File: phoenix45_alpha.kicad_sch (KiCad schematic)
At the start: 115 parts, among them J1 AVR-ISP-6, SW1 SW_PUSH, SW2 SW_PUSH, U1 SRV05-4, U3 ATmega32U4-M, X1 Crystal_GND24_Small

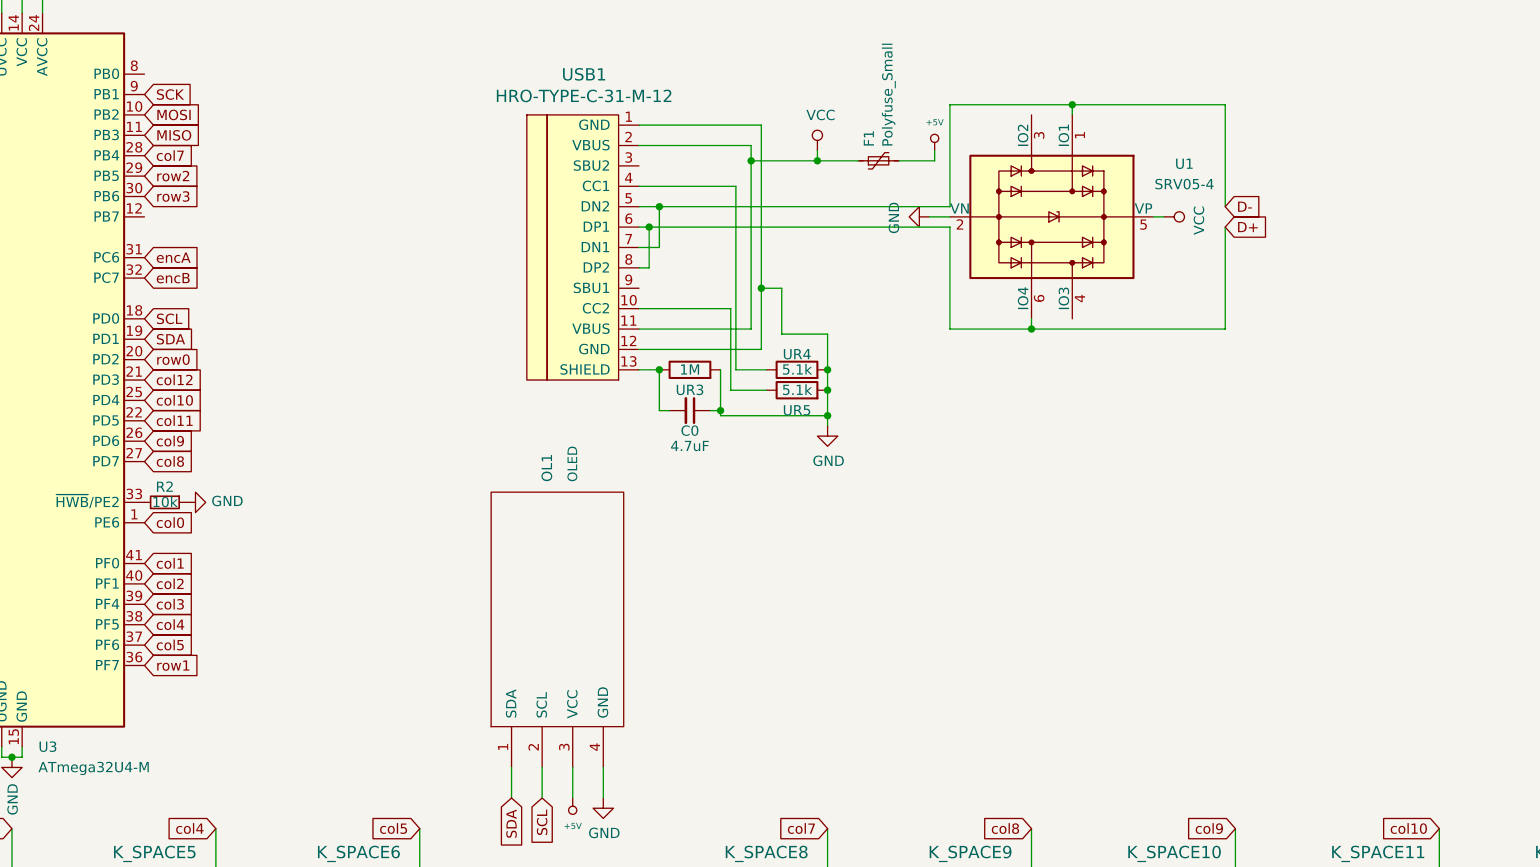
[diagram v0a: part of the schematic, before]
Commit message: trackpoint
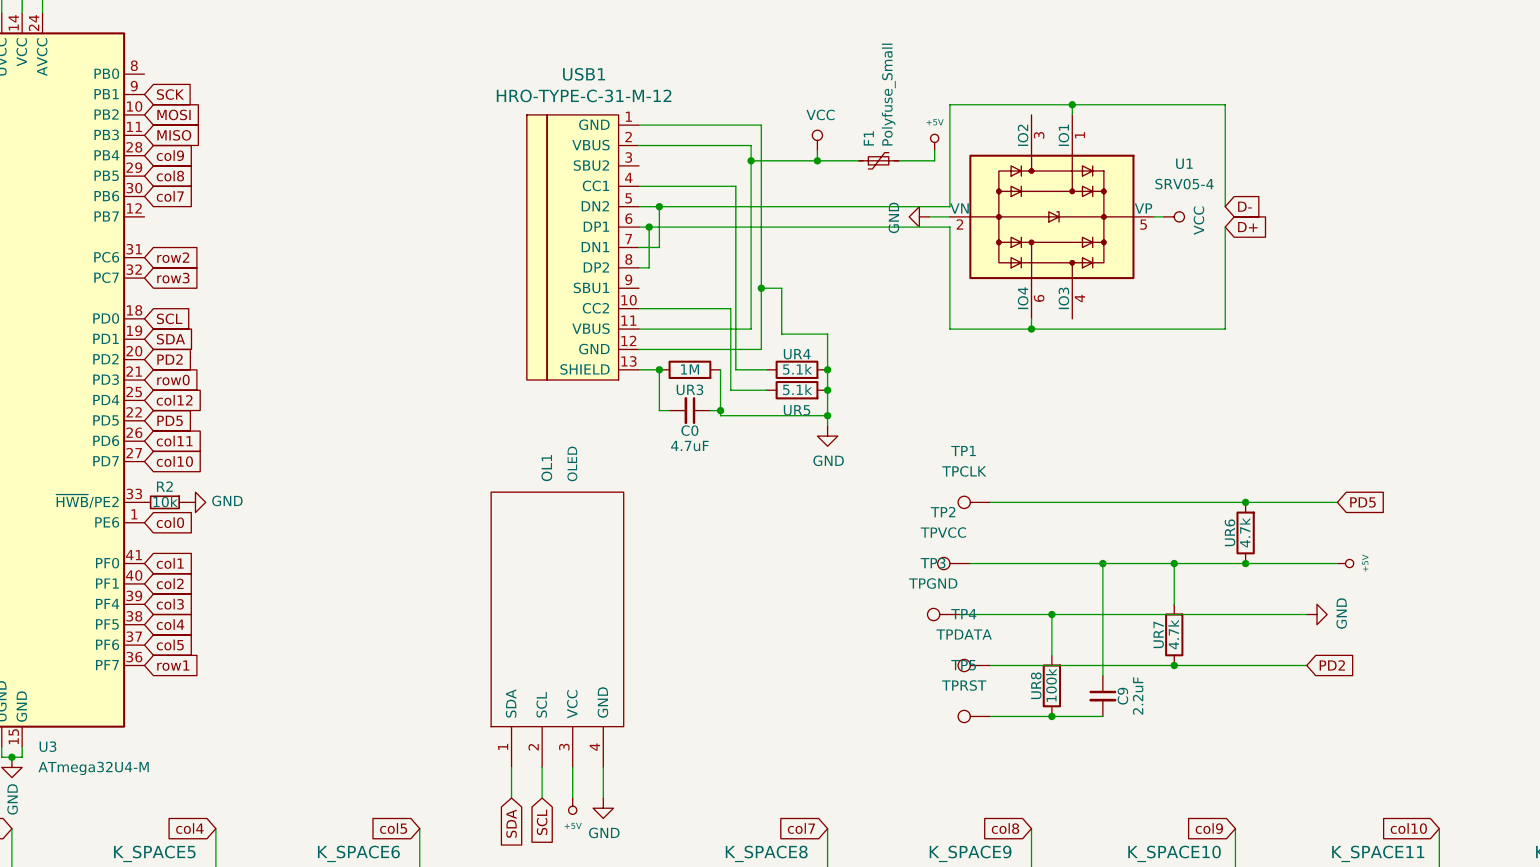
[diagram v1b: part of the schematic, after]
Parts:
- added C9: 2.2uF, Capacitor_SMD:C_0805_2012Metric_Pad1.18x1.45mm_HandSolder, symbol device:C_Small
- added TP1: TPCLK, TestPoint:TestPoint_Pad_1.0x1.0mm, symbol Connector:TestPoint
- added TP2: TPVCC, TestPoint:TestPoint_Pad_1.0x1.0mm, symbol Connector:TestPoint
- added TP3: TPGND, TestPoint:TestPoint_Pad_1.0x1.0mm, symbol Connector:TestPoint
- added TP4: TPDATA, TestPoint:TestPoint_Pad_1.0x1.0mm, symbol Connector:TestPoint
- added TP5: TPRST, TestPoint:TestPoint_Pad_1.0x1.0mm, symbol Connector:TestPoint
- added UR6, UR7: 4.7k, Resistor_SMD:R_0805_2012Metric_Pad1.20x1.40mm_HandSolder, symbol device:R
- added UR8: 100k, Resistor_SMD:R_0805_2012Metric_Pad1.20x1.40mm_HandSolder, symbol device:R
- C0, C1, C2, C3, C4, C5, C6, C7, C8: footprint Capacitor_SMD:C_0805_2012Metric -> Capacitor_SMD:C_0805_2012Metric_Pad1.18x1.45mm_HandSolder
- R1, R2, UR1, UR2, UR3, UR4, UR5: footprint Resistor_SMD:R_0805_2012Metric -> Resistor_SMD:R_0805_2012Metric_Pad1.20x1.40mm_HandSolder
- U1: footprint Package_TO_SOT_SMD:SOT-23-6 -> Package_TO_SOT_SMD:SOT-23-6_Handsoldering
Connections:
- net encA is gone; now on net row2: U3.31 (PC6)
- net encB is gone; now on net row3: U3.32 (PC7)
- net +5V: now also C9.1, TP2.1, UR6.1, UR7.2
- net GND: now also TP3.1, UR8.2
- net col10: now also U3.27 (PD7); no longer U3.25 (PD4)
- net col11: now also U3.26 (PD6); no longer U3.22 (PD5)
- net col12: now also U3.25 (PD4); no longer U3.21 (PD3)
- net col7: now also U3.30 (PB6); no longer U3.28 (PB4)
- net col8: now also U3.29 (PB5); no longer U3.27 (PD7)
- net col9: now also U3.28 (PB4); no longer U3.26 (PD6)
- net row0: now also U3.21 (PD3); no longer U3.20 (PD2)
- net row2: no longer U3.29 (PB5)
- net row3: no longer U3.30 (PB6)
- new net: C9.2, TP5.1, UR8.1
- new net PD2: TP4.1, U3.20 (PD2), UR7.1
- new net PD5: TP1.1, U3.22 (PD5), UR6.2
